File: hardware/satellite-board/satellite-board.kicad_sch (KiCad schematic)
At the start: 27 parts, among them J1 MTJ-88ARX1-FSM-LG, J2 B2B-PH-K-S, Q1 2N7002, U1 LORA1262-915TCXO, U2 XC6220B331MR, U3 ESP32-C6-DEVKITC-1-N8, U4 MAX3485

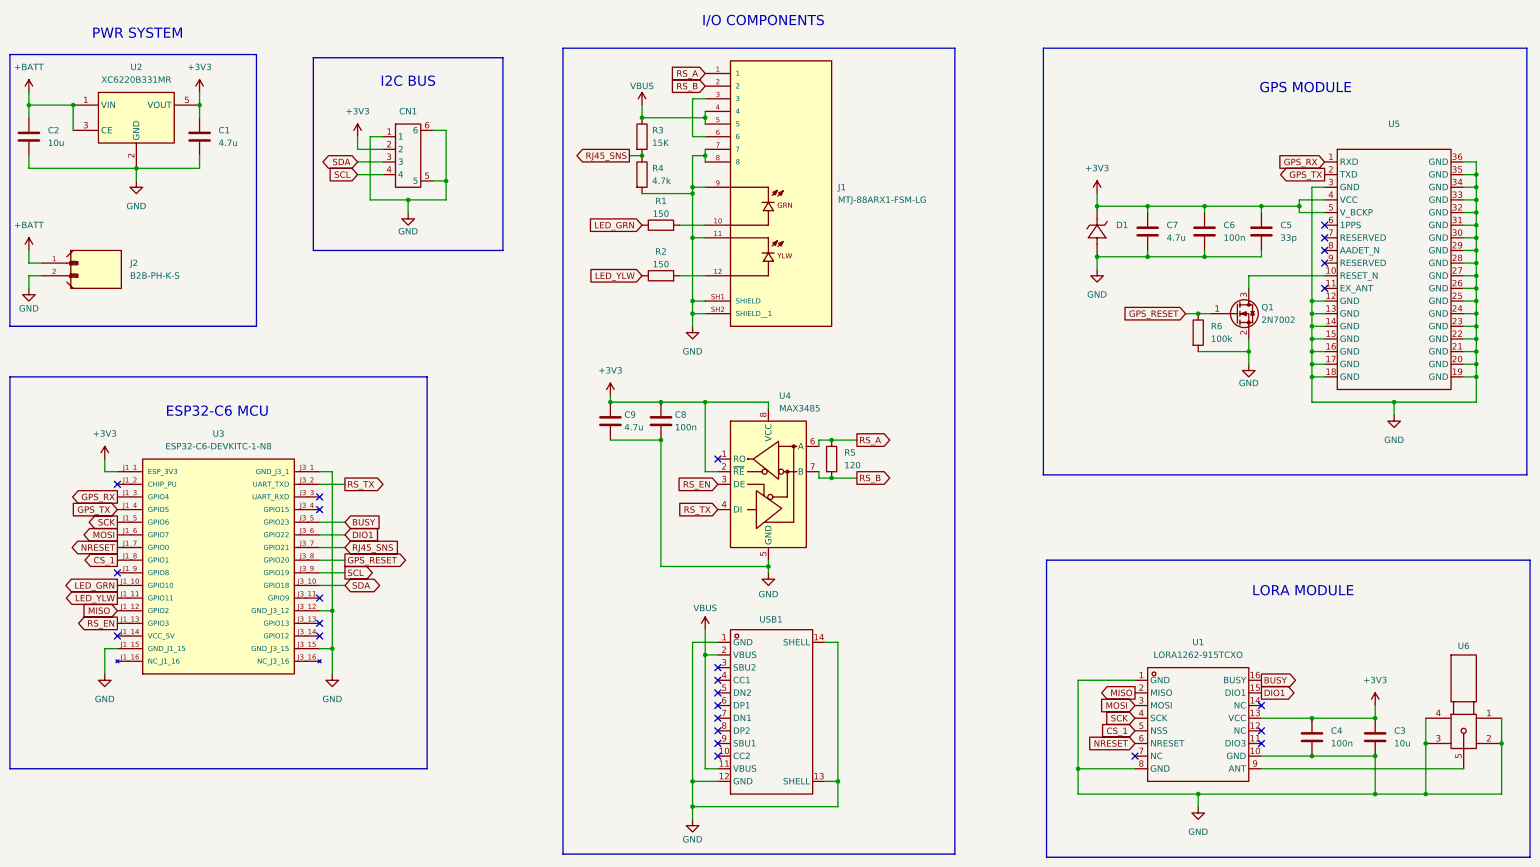
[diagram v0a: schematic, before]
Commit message: Satelite Board Started
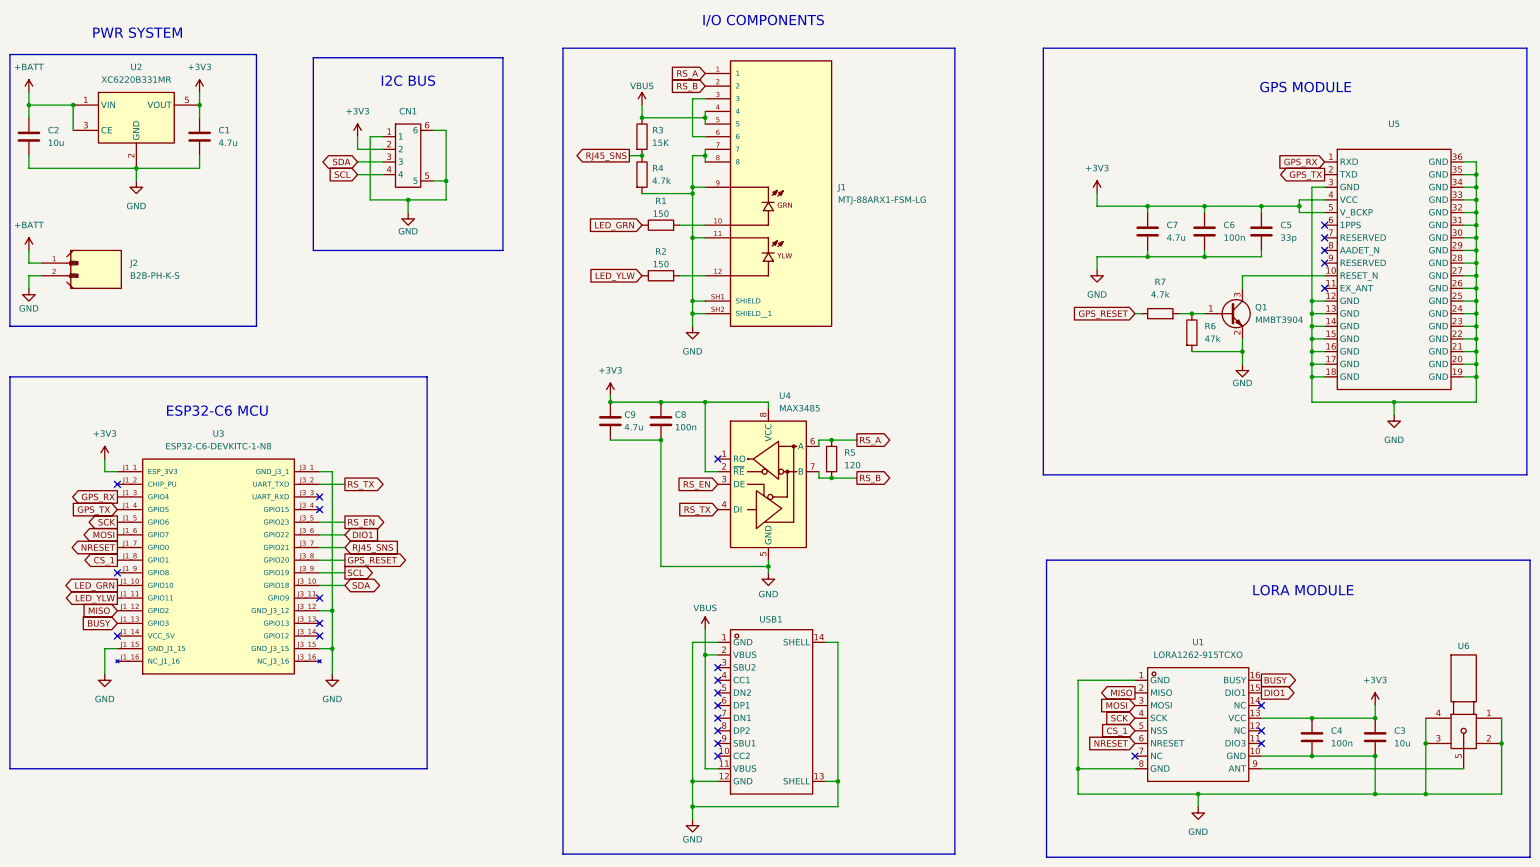
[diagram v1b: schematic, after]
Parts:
- removed D1: ~, Diode_SMD:D_SOD-323F, symbol 5678:PESD3V3L1UA_C7588061
- removed Q1: 2N7002, Package_TO_SOT_SMD:SOT-23, symbol Transistor_FET:2N7002
- added Q1: MMBT3904, Package_TO_SOT_SMD:SOT-23, symbol Transistor_BJT:MMBT3904
- added R7: 4.7k, Resistor_SMD:R_0402_1005Metric, symbol Device:R
- R6: value 100k -> 47k; LCSC C25741 -> C25792
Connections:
- net BUSY: now also U3.J1_13 (GPIO3); no longer U3.J3_5 (GPIO23)
- net GND: now also Q1.2 (E)
- net GPS_RESET: now also R7.1; no longer R6.1
- net RS_EN: now also U3.J3_5 (GPIO23); no longer U3.J1_13 (GPIO3)
- net at U5.10 (RESET_N): now also Q1.3 (C)
- new net: Q1.1 (B), R6.1, R7.2
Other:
- moved on the sheet: R6

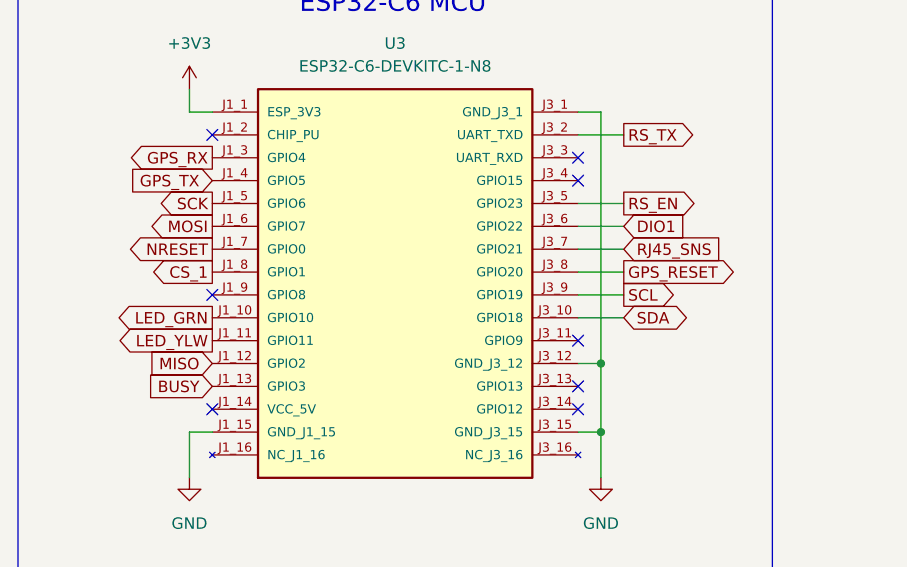
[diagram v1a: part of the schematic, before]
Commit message: Updates to Sat
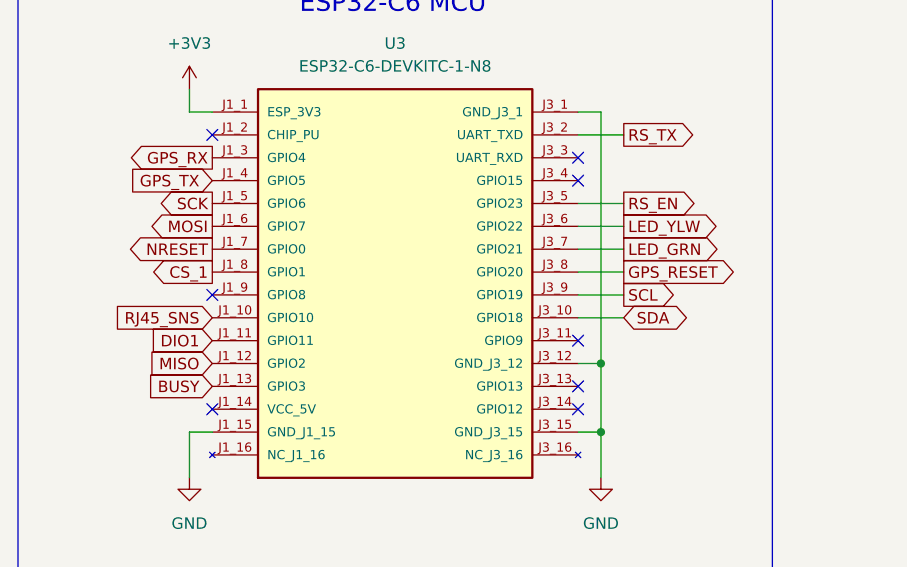
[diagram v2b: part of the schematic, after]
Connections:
- net DIO1: now also U3.J1_11 (GPIO11); no longer U3.J3_6 (GPIO22)
- net LED_GRN: now also U3.J3_7 (GPIO21); no longer U3.J1_10 (GPIO10)
- net LED_YLW: now also U3.J3_6 (GPIO22); no longer U3.J1_11 (GPIO11)
- net RJ45_SNS: now also U3.J1_10 (GPIO10); no longer U3.J3_7 (GPIO21)
